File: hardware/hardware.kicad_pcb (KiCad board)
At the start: 2 copper layers, 39 parts, among them J1 USB_C_Receptacle_USB2.0, J2 Conn_01x12_Pin, J4 Conn_01x12_Pin, SW1 RST, SW2 BOOT, U1 ESP32-C3-MINI-1, U2 CH217K, U3 AMS1117-3.3, U4 DHT11, U5 BMP280, U6 BH1750FVI

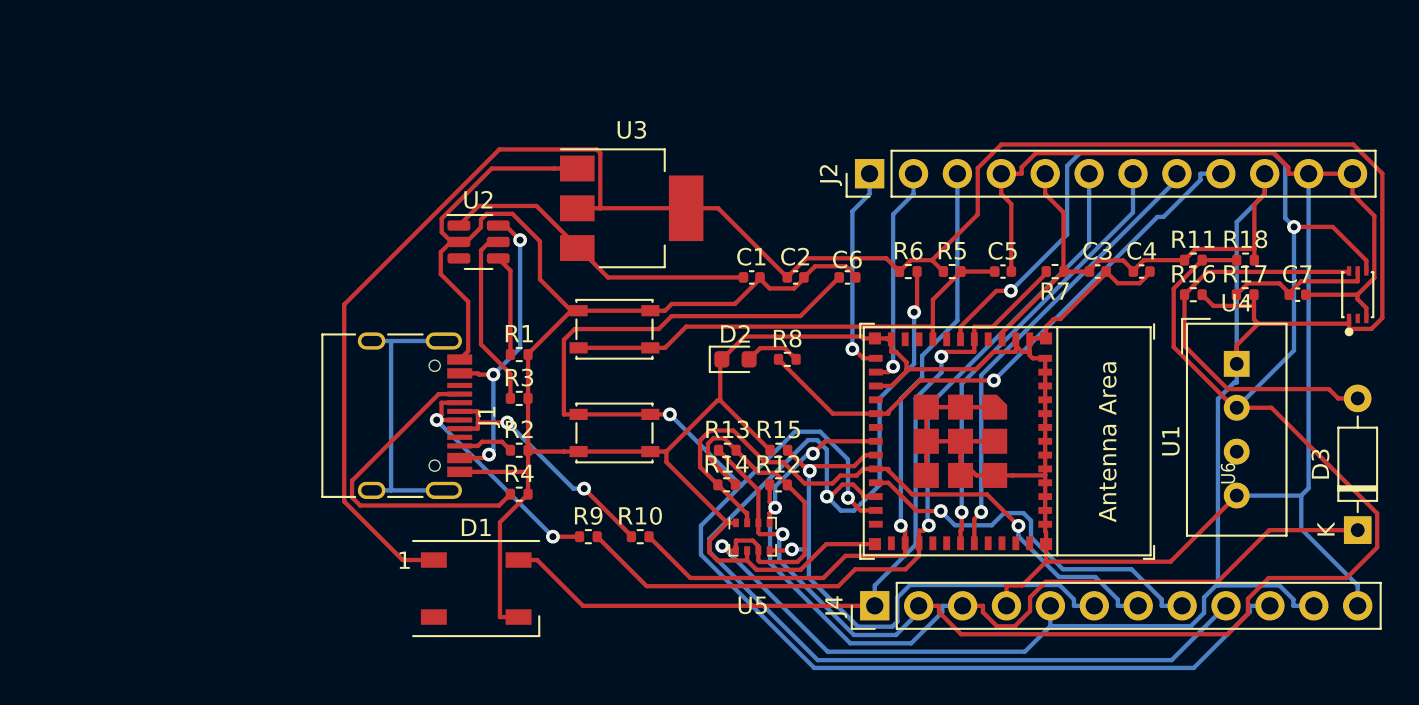
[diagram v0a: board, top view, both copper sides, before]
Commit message: PCB is ready for print.
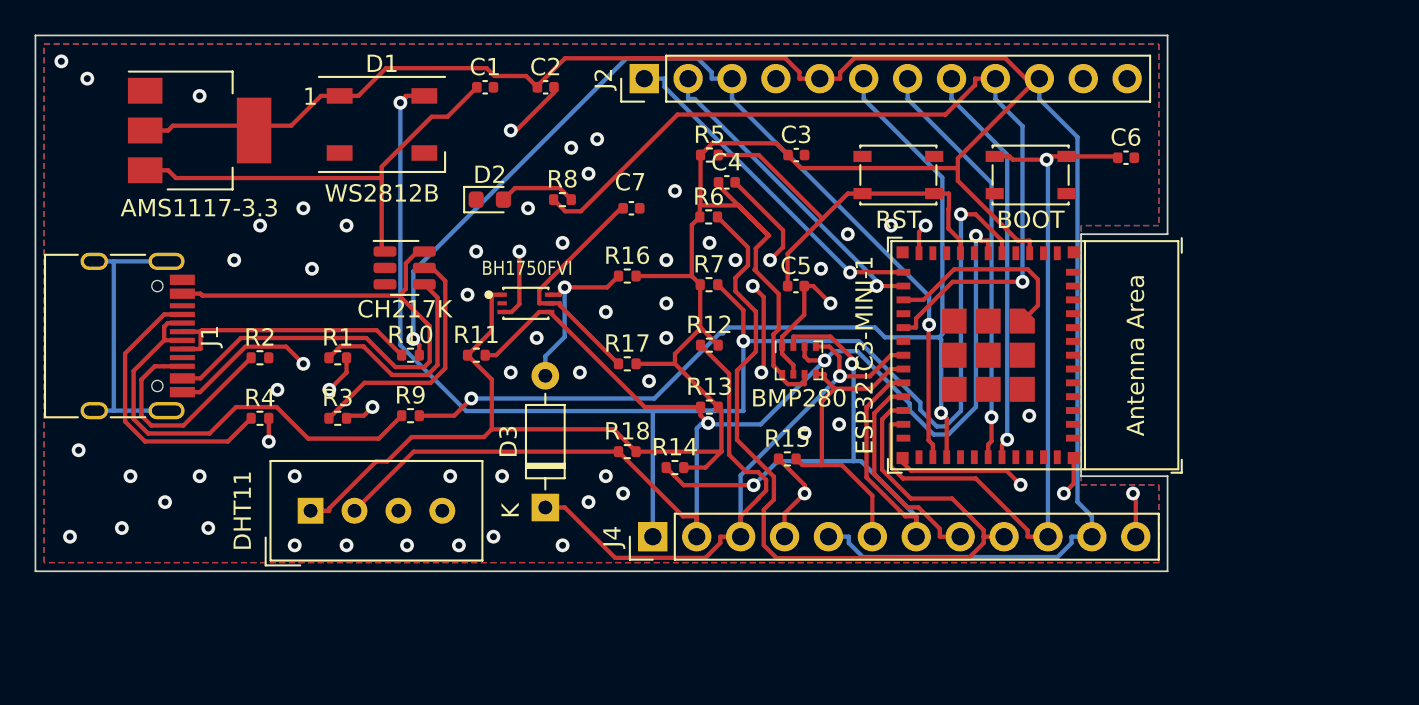
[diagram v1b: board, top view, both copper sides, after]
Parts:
- moved U4 54.3 mm to (145.4, 87.5), turned to 90 degrees
- moved U6 48.1 mm to (157.9, 75.5), turned to 0 degrees
- moved D3 47.0 mm to (159.0, 87.3)
- moved R11 41.8 mm to (155.0, 78.5)
- moved C7 38.9 mm to (164.0, 70.0)
- moved R18 37.4 mm to (163.7, 84.1)
- moved R17 36.0 mm to (163.7, 79.0)
- moved R16 32.8 mm to (163.7, 73.9)
- moved SW2 28.3 mm to (187.1, 68.1)
- moved D1 27.4 mm to (149.6, 65.2)
- moved U3 25.4 mm to (139.0, 65.5)
- moved C4 24.5 mm to (169.5, 68.5)
- moved R7 20.0 mm to (168.5, 74.4), turned to 0 degrees
- moved C1 18.9 mm to (155.5, 63.0)
- moved C3 18.7 mm to (173.5, 66.9)
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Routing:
- net GND: track 263.9 -> 72.4 mm, vias 0 -> 67
- net IO9_BOOT: track 88.3 -> 43.3 mm, vias 2 -> 1
- net IO3_SDA: track 122.5 -> 81.4 mm
- net IO2: track 46.7 -> 82.6 mm, vias 1 -> 3
- net IO8: track 67.4 -> 49.1 mm, vias 2 -> 0
- net 3V3: track 234.0 -> 215.8 mm, vias 1 -> 0
- net Net-(U2-VIN): track 18.5 -> 36.6 mm, vias 3 -> 0
- net IO10: track 32.9 -> 49.9 mm
- net IO5: track 34.7 -> 18.4 mm, vias 2 -> 0
- net IO18: track 39.9 -> 56.0 mm, vias 1 -> 2
- net Net-(D3-A): track 24.3 -> 10.1 mm, vias 0 -> 1
- net USBD-: track 14.6 -> 26.1 mm, vias 2 -> 0
- net Net-(J1-CC2): track 3.24 -> 13.0 mm
- net IO7: track 22.0 -> 12.3 mm, vias 1 -> 0
- net IO19: track 46.9 -> 56.5 mm, vias 1 -> 2
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- added copper zone on B.Cu, net GND
- added copper zone on F.Cu, net GND
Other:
- board outline added: 65.5 x 31 mm
